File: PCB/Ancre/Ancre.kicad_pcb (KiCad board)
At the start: 2 copper layers, 78.9 x 74 mm, 17 parts, among them IC1 TCAN1051VDRQ1, U1 OKI-78SR-5_1.5-W36-C, U2 DB301V-5.0-2P, U3 DB301V-5.0-2P, U6 DB301V-5.0-2P, U7 DB301V-5.0-2P

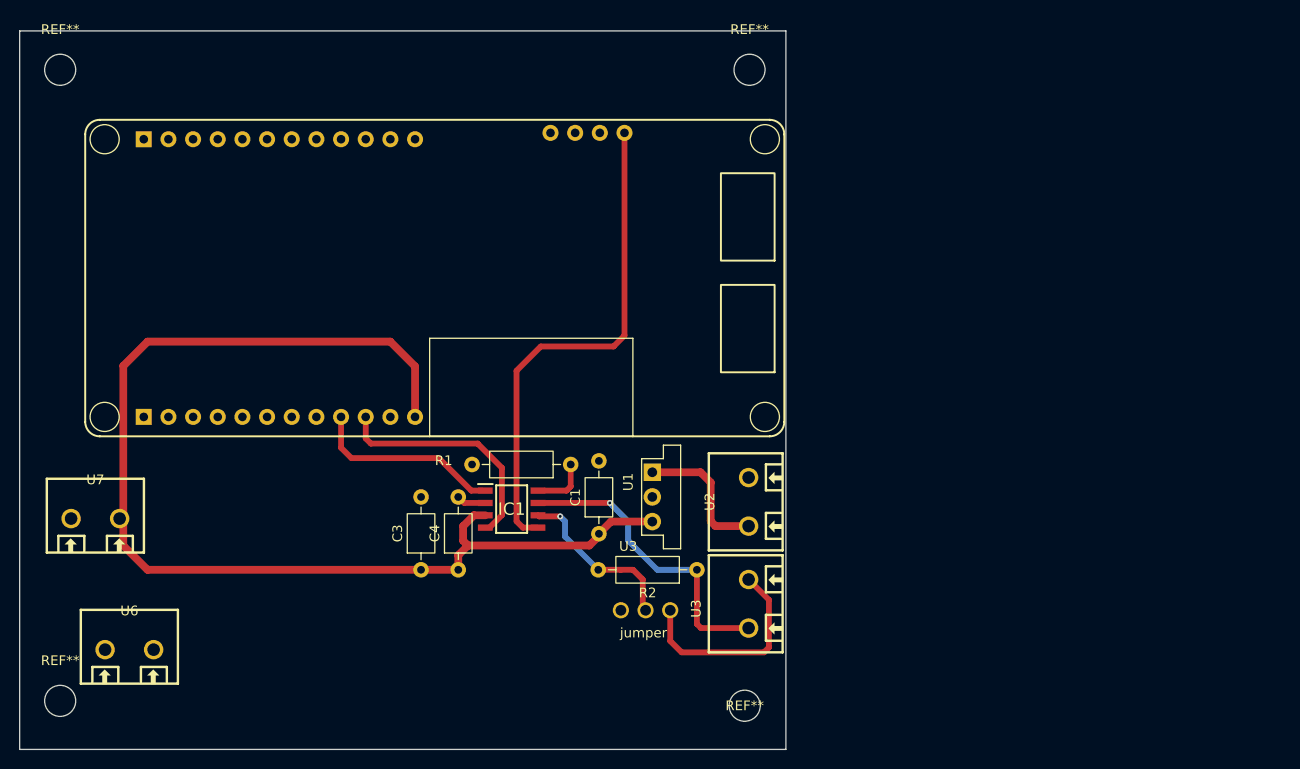
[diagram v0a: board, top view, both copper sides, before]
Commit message: MaJ PCB Ancre
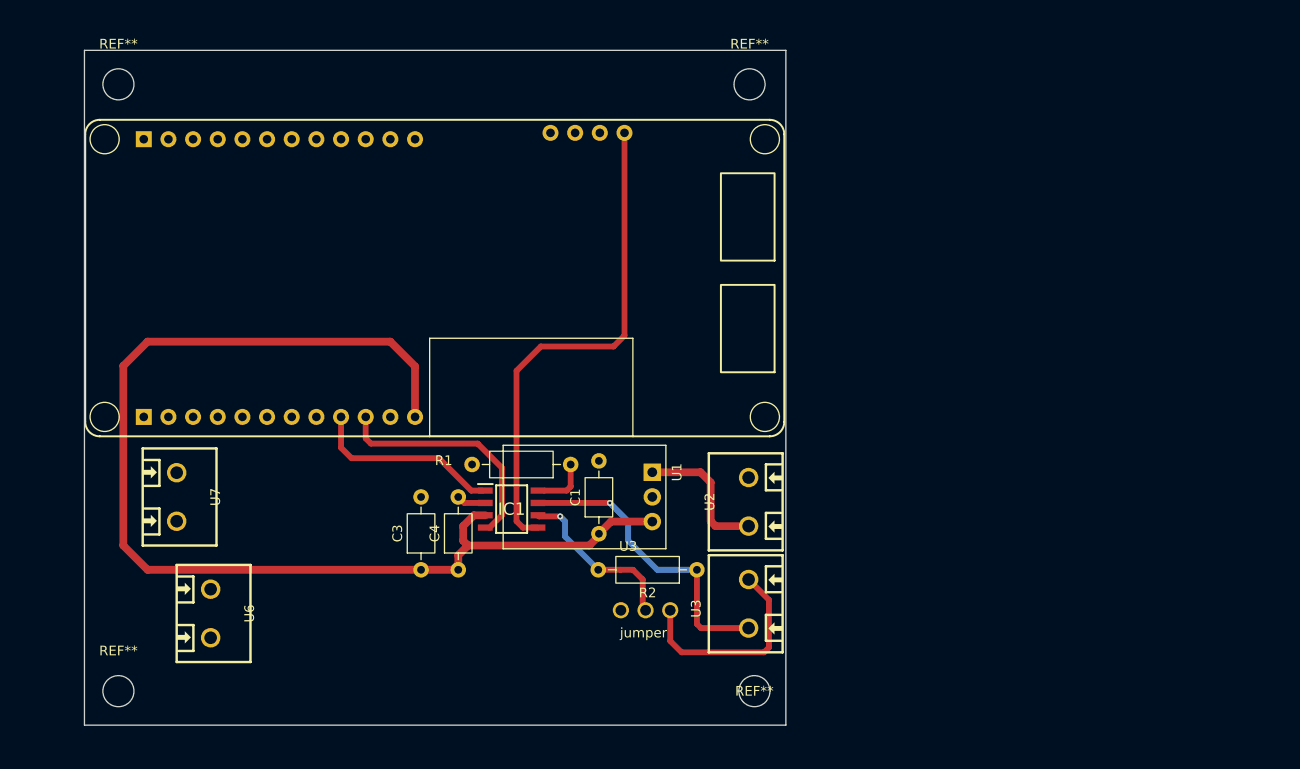
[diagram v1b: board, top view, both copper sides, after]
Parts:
- U1: footprint Converter_DCDC:Converter_DCDC_Murata_OKI-78SR_Vertical -> Bibliotheque_Projet:Abaisseur 5v OKI
- moved U6 9.17 mm to (163.5, 93.0), turned to -90 degrees
- moved U7 8.67 mm to (160.0, 81.0), turned to -90 degrees
- moved REF** 6.18 mm to (154.0, 38.5)
- moved REF** 6.08 mm to (154.0, 101.0)
- moved REF** 1.80 mm to (219.5, 101.0)
- moved REF** 1.50 mm to (219.0, 38.5)
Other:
- board size 78.9 x 74 mm -> 72.2 x 69.5 mm

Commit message: finalisation PCB ancre
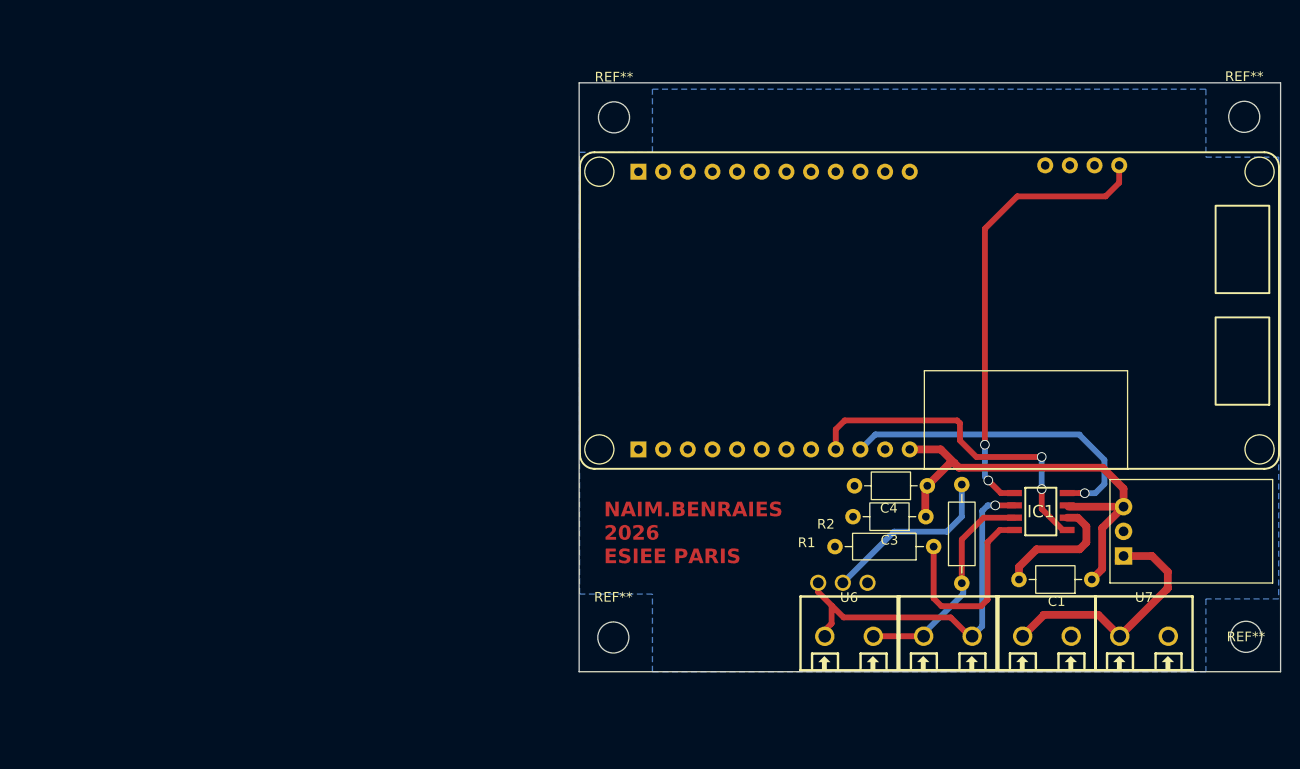
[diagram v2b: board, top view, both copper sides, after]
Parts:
- moved U7 100.7 mm to (259.6, 95.3), turned to 0 degrees
- moved U6 65.8 mm to (229.2, 95.3), turned to 0 degrees
- moved IC1 54.5 mm to (249.0, 82.5), turned to 180 degrees
- moved C3 52.3 mm to (237.2, 83.0), turned to 180 degrees
- moved REF** 51.3 mm to (205.0, 95.5)
- moved REF** 51.2 mm to (205.0, 41.9)
- moved REF** 51.1 mm to (270.0, 41.8)
- moved U4 51.1 mm to (231.4, 63.6)
- moved C1 51.0 mm to (254.2, 89.5), turned to 180 degrees
- moved REF** 50.9 mm to (270.1, 95.4)
- moved U1 49.3 mm to (257.5, 87.1), turned to 90 degrees
- moved C4 49.1 mm to (237.3, 79.8), turned to 180 degrees
- moved R1 38.3 mm to (238.0, 86.1)
- moved U5 35.4 mm to (236.1, 89.8), turned to -90 degrees
- moved U2 33.7 mm to (249.6, 95.3), turned to 0 degrees
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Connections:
- R2 pad 2: Net-(IC1-CANL) -> Net-(U5-Resistance)
- U3 pad 2: Net-(U5-CAN_line) -> Net-(IC1-CANL)
- U5 pad J1: Net-(IC1-CANL) -> Net-(U5-Resistance)
- U5 pad J2: Net-(U5-CAN_line) -> Net-(IC1-CANL)
- U6 pad 1: Net-(IC1-CANH) -> Net-(IC1-CANL)
- U6 pad 2: Net-(U5-CAN_line) -> Net-(IC1-CANH)
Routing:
- net +5V: track 119.4 -> 47.5 mm
- net Net-(U5-CAN_line): track 21.9 -> 0.00 mm
- net Net-(IC1-CANL): track 18.4 -> 39.0 mm
- net Net-(U5-Resistance): track 0.00 -> 18.6 mm
- net Net-(IC1-TXD): track 19.9 -> 35.1 mm, vias 0 -> 2
- net Net-(IC1-S): track 5.81 -> 20.7 mm
- net +12V: track 15.3 -> 26.7 mm
- net GNDREF: track 3.04 -> 13.3 mm
- net Net-(IC1-RXD): track 24.6 -> 33.6 mm, vias 0 -> 1
- net Net-(IC1-CANH): track 32.6 -> 23.8 mm, vias 1 -> 0
- net Net-(IC1-NC): track 51.5 -> 46.9 mm, vias 0 -> 2
- added copper zone on B.Cu, net GNDREF
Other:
- board size 72.2 x 69.5 mm -> 72.2 x 60.7 mm
- board text added: "NAIM.BENRAIES 2026 ESIEE PARIS"
